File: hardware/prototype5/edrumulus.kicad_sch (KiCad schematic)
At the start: 87 parts, among them J1 Trigger Connector, J2 Raspberry Pi GPIO pins, U1 ESP32-WROOM-32U, U2 AMS1117-3.3, U3 MCP1754S-3302xMB

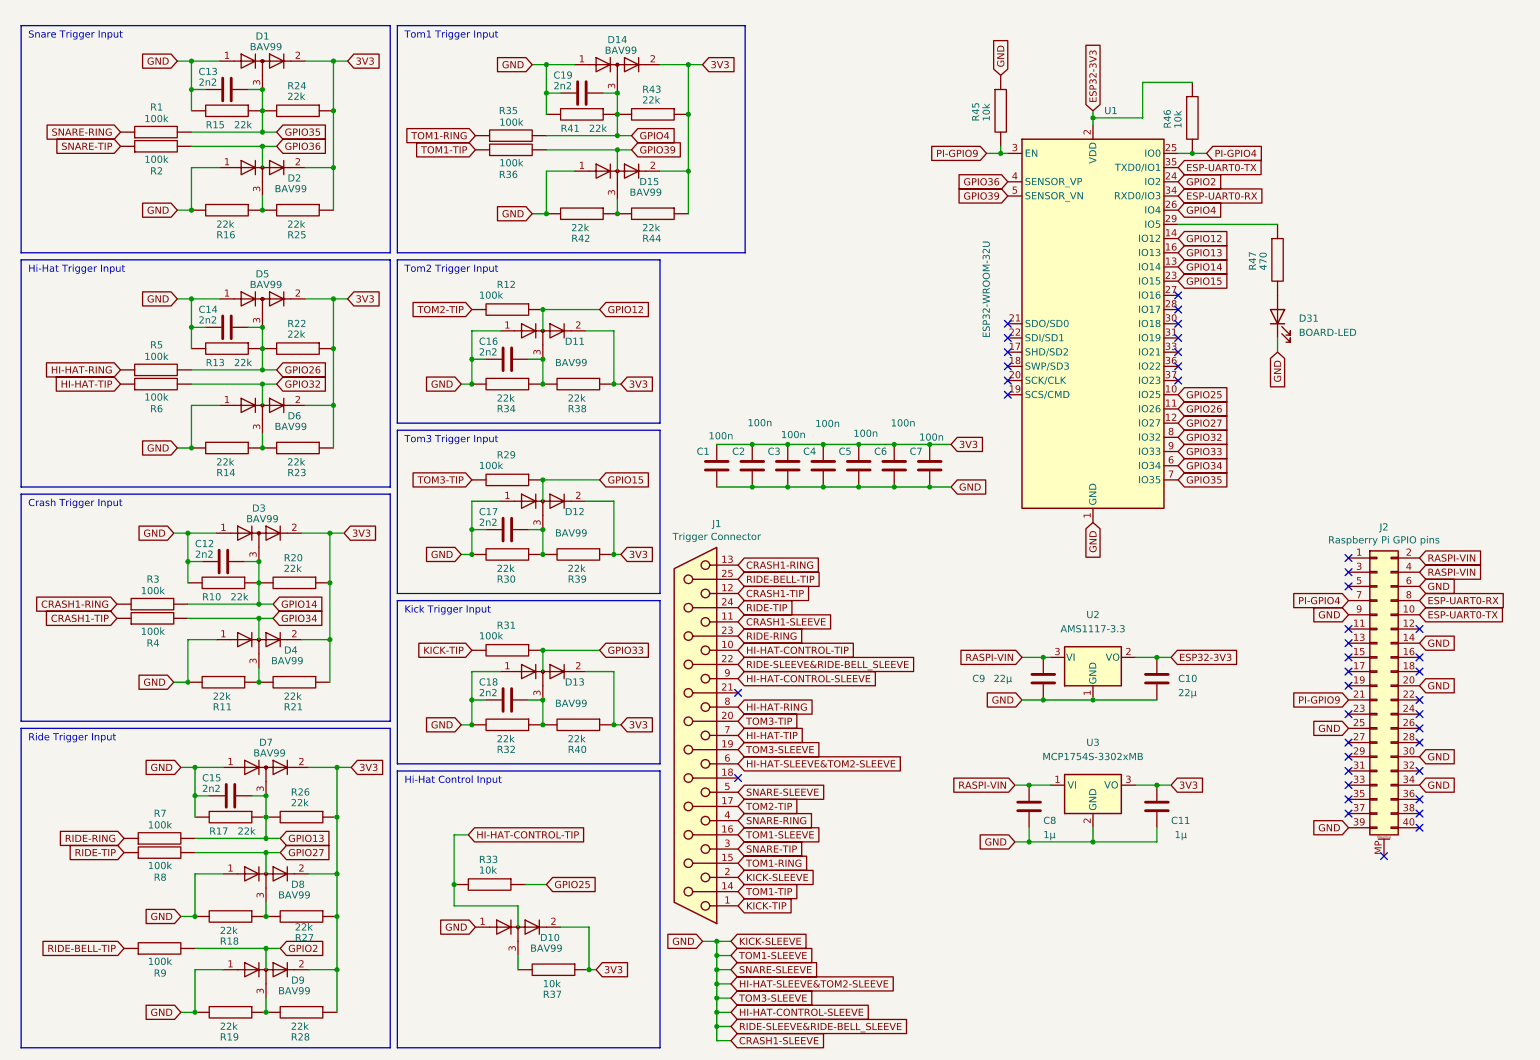
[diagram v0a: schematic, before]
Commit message: delivery jstma for prototype 5 on 8/24/2022
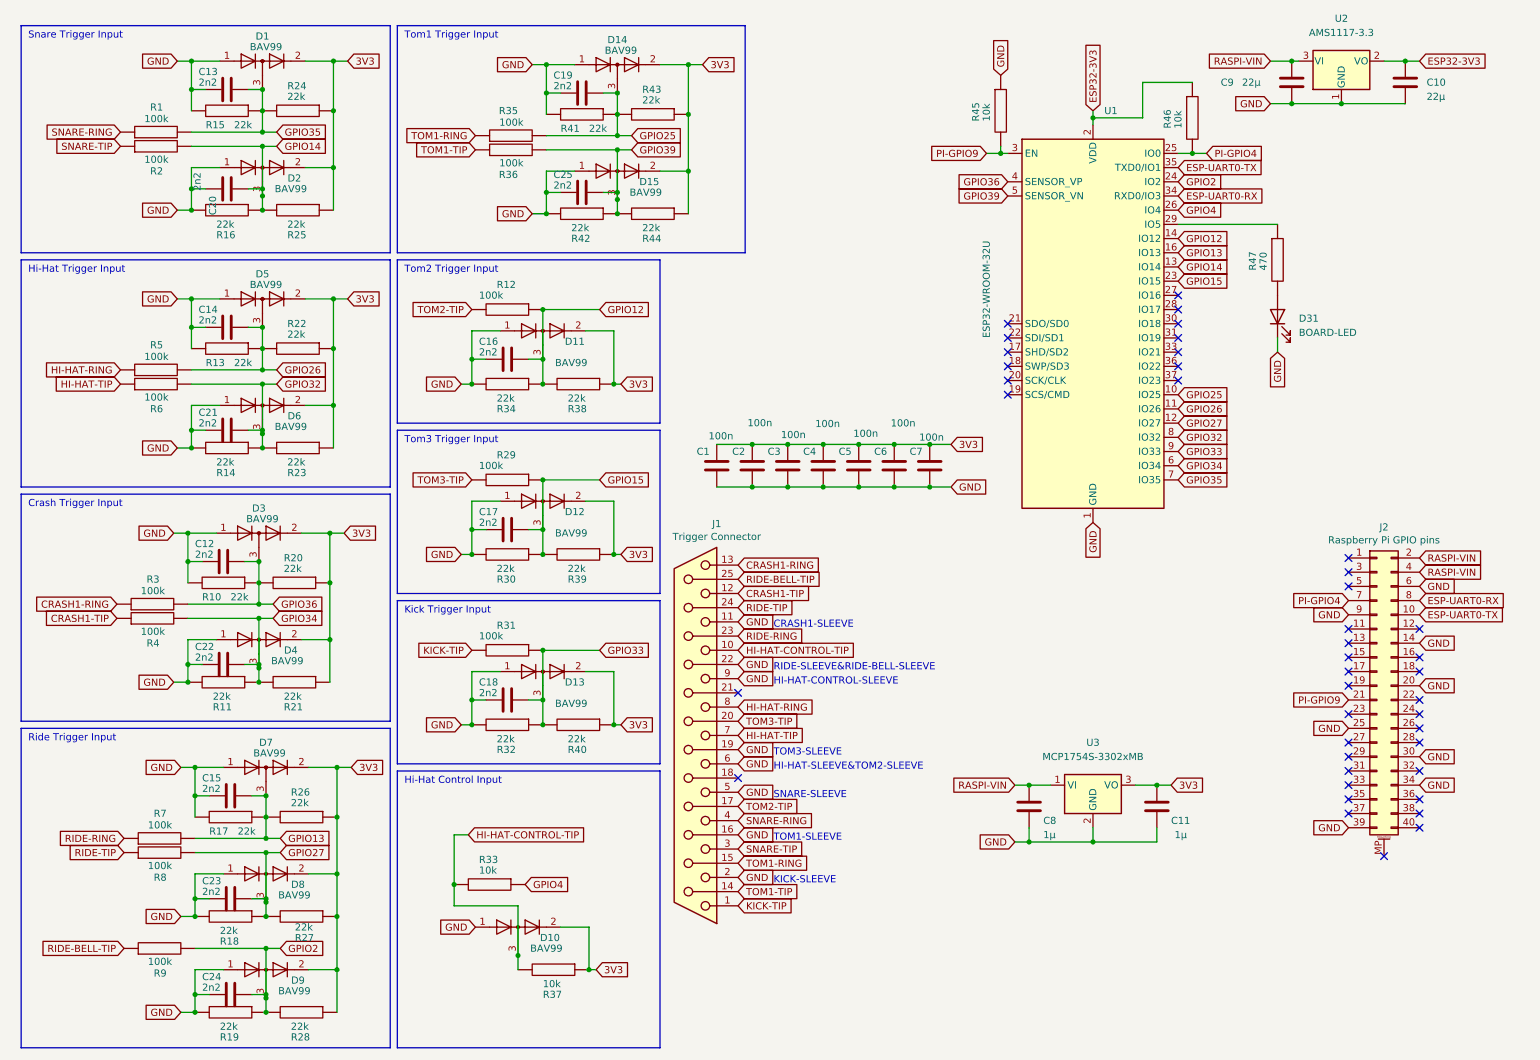
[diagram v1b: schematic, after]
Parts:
- added C20, C21, C22, C23, C24, C25: 2n2, Capacitor_SMD:C_0603_1608Metric_Pad1.08x0.95mm_HandSolder, symbol Device:C
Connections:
- net GPIO12: now also C16.1, D11.3 (K), R34.1, R38.2
- net GPIO14: now also D2.3 (K), R16.1, R2.2, R25.2, C20.1; no longer C12.1, D3.3 (K), R10.1, R20.2, R3.2
- net GPIO15: now also C17.1, D12.3 (K), R30.1, R39.2
- net GPIO2: now also D9.3 (K), R19.1, R28.2, C24.1
- net GPIO25: now also C19.1, D14.3 (K), R35.2, R41.1, R43.2; no longer R33.1
- net GPIO27: now also D8.3 (K), R18.1, R27.2, C23.1
- net GPIO32: now also D6.3 (K), R14.1, R23.2, C21.1
- net GPIO33: now also C18.1, D13.3 (K), R32.1, R40.2
- net GPIO34: now also D4.3 (K), R11.1, R21.2, C22.1
- net GPIO36: now also C12.1, D3.3 (K), R10.1, R20.2, R3.2; no longer R2.2
- net GPIO39: now also D15.3 (K), R42.1, R44.2, C25.1
- net GPIO4: now also R33.1; no longer C19.1, D14.3 (K), R35.2, R41.1, R43.2
- net HI-HAT-CONTROL-TIP: now also D10.3 (K), R37.2
- net CRASH1-SLEEVE renamed GND
- net GND: now also C20.2, C21.2, C22.2, C23.2, C24.2, C25.2
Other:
- note added: "CRASH1-SLEEVE"
- note added: "HI-HAT-CONTROL-SLEEVE"
- note added: "HI-HAT-SLEEVE&TOM2-SLEEVE"
- note added: "KICK-SLEEVE"
- note added: "RIDE-SLEEVE&RIDE-BELL-SLEEVE"
- note added: "SNARE-SLEEVE"
- note added: "TOM1-SLEEVE"
- note added: "TOM3-SLEEVE"
- moved on the sheet: C10, C9, U2
